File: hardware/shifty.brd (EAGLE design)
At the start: 35.2 x 43.2 mm, 15 parts, among them IC1 74HC595D, IC2 74HC595D, IC3 ULN2003AD, IC4 ULN2003AD

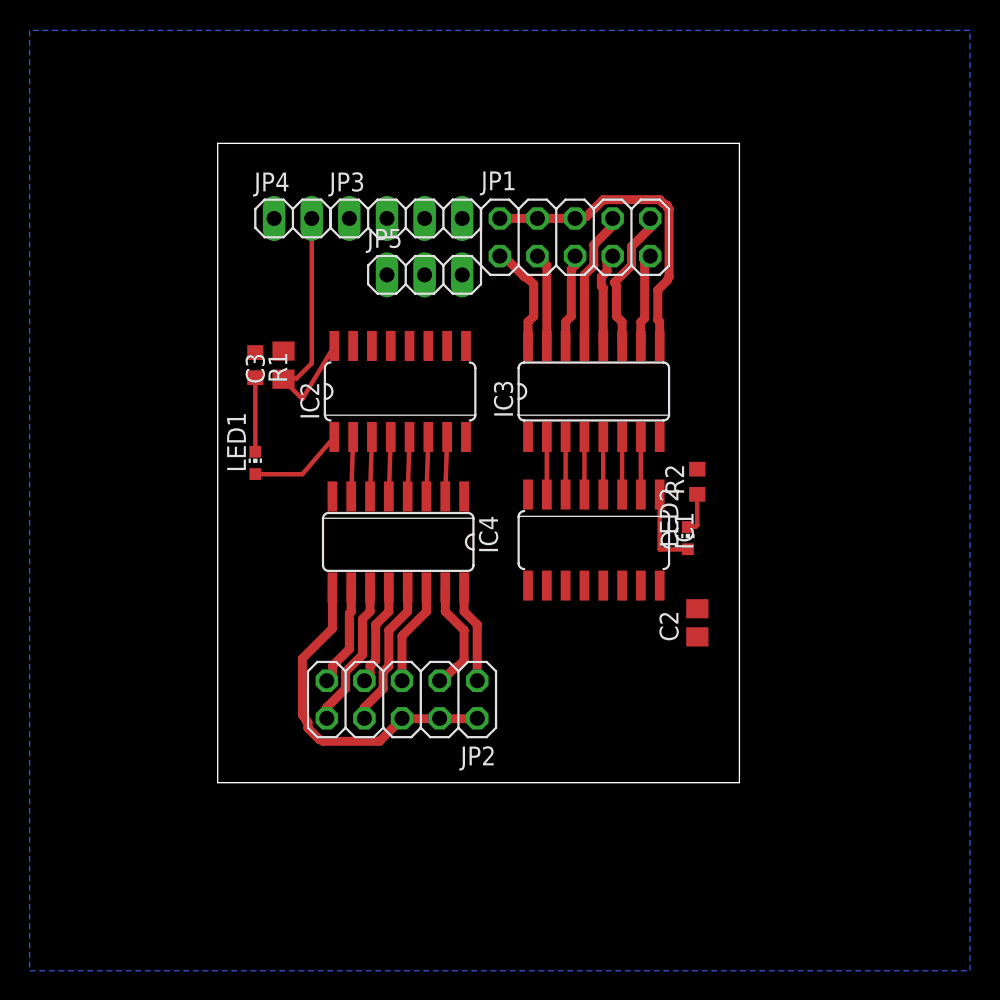
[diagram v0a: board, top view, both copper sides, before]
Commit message: Board lay-out done
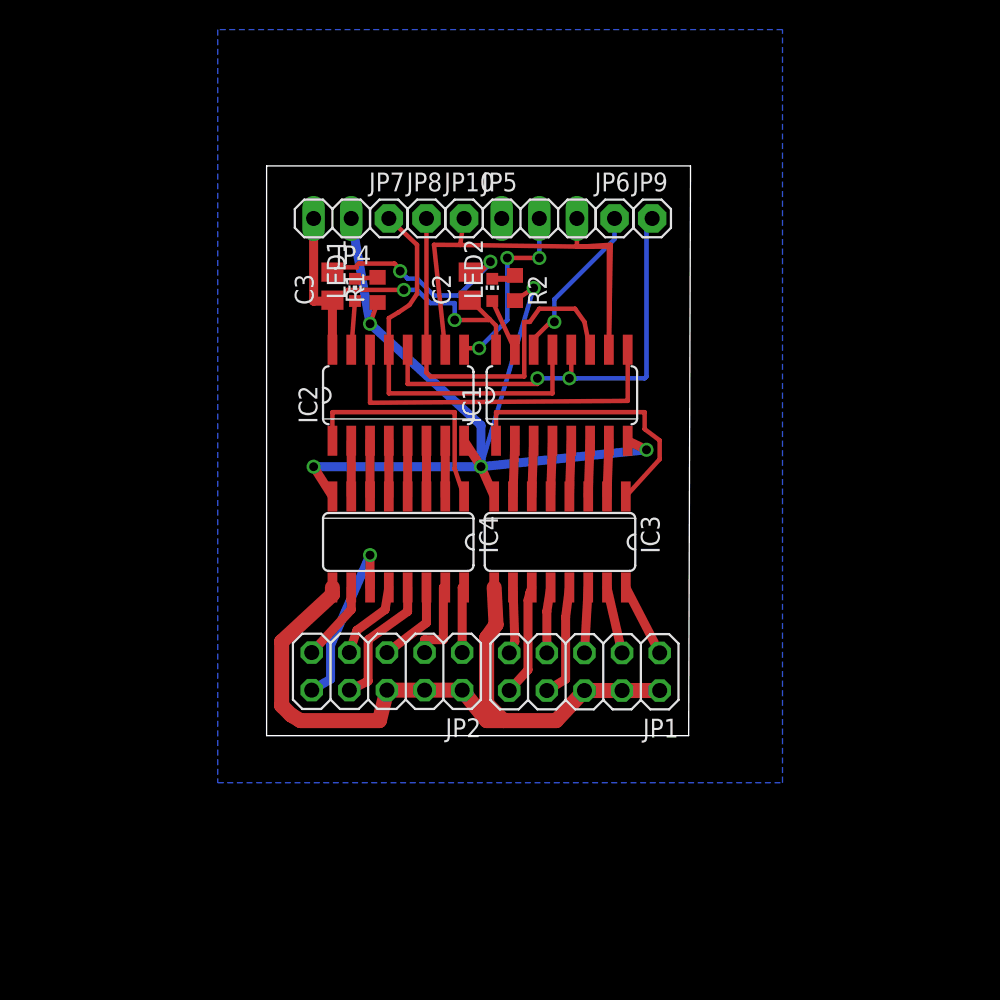
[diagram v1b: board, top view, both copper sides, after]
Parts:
- removed JP3: (no value), pinhead:1X04
- added JP10, JP6, JP7, JP8, JP9: (no value), adafruit:1X01
- moved JP1 29.3 mm to (24.8, 7.49), turned to 180 degrees
- moved C2 27.4 mm to (17.0, 33.5)
- moved LED2 21.3 mm to (18.5, 33.3)
- moved R2 18.0 mm to (20.1, 33.4), turned to 270 degrees
- moved LED1 13.5 mm to (9.27, 33.3)
- moved IC3 10.4 mm to (23.1, 16.3), turned to 180 degrees
- moved IC1 10.0 mm to (23.2, 26.2), turned to 0 degrees
- moved R1 9.69 mm to (10.8, 33.3), turned to 90 degrees
- moved JP5 8.63 mm to (21.7, 38.1)
- moved C3 6.27 mm to (7.75, 33.5)
- moved JP4 2.67 mm to (7.75, 38.1), turned to 180 degrees
- moved JP2 2.16 mm to (11.4, 7.52)
- moved IC2 0.28 mm to (12.2, 26.2)
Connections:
- net N$1: now also IC1.1; no longer IC1.15
- net N$16: now also JP6.1; no longer JP3.4
- net N$17: now also IC2.15; no longer IC2.1
- net N$18: now also JP10.1
- net N$20: now also JP9.1; no longer JP3.1
- net N$38: now also IC1.15; no longer IC1.1
- net N$43: now also JP7.1; no longer JP3.3
- net N$8: now also JP8.1; no longer JP3.2
- net N$9: now also IC2.1; no longer IC2.15
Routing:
- net GND: track 0.00 -> 66.9 mm, vias 0 -> 5
- net N$18: track 0.00 -> 39.0 mm
- net N$20: track 0.00 -> 31.7 mm, vias 0 -> 2
- net N$8: track 0.00 -> 27.7 mm
- net N$43: track 0.00 -> 27.6 mm
- net N$19: track 0.00 -> 24.4 mm
- net N$1: track 0.00 -> 19.0 mm
- net N$9: track 0.00 -> 16.0 mm
- net GNDIO: track 0.00 -> 15.2 mm, vias 0 -> 2
- net N$29: track 0.00 -> 12.8 mm, vias 0 -> 3
- net N$16: track 0.00 -> 11.3 mm, vias 0 -> 1
- net VCC: track 18.2 -> 27.2 mm, vias 0 -> 2
- net N$28: track 5.34 -> 1.53 mm
- net +10V: track 44.8 -> 48.5 mm
- net N$17: track 6.50 -> 3.30 mm
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- added copper zone on layer 16, net N$39
- removed copper zone on layer 16, net GND
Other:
- board size 35.2 x 43.2 mm -> 28.6 x 38.5 mm
